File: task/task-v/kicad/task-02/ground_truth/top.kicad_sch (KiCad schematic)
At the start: 0 parts

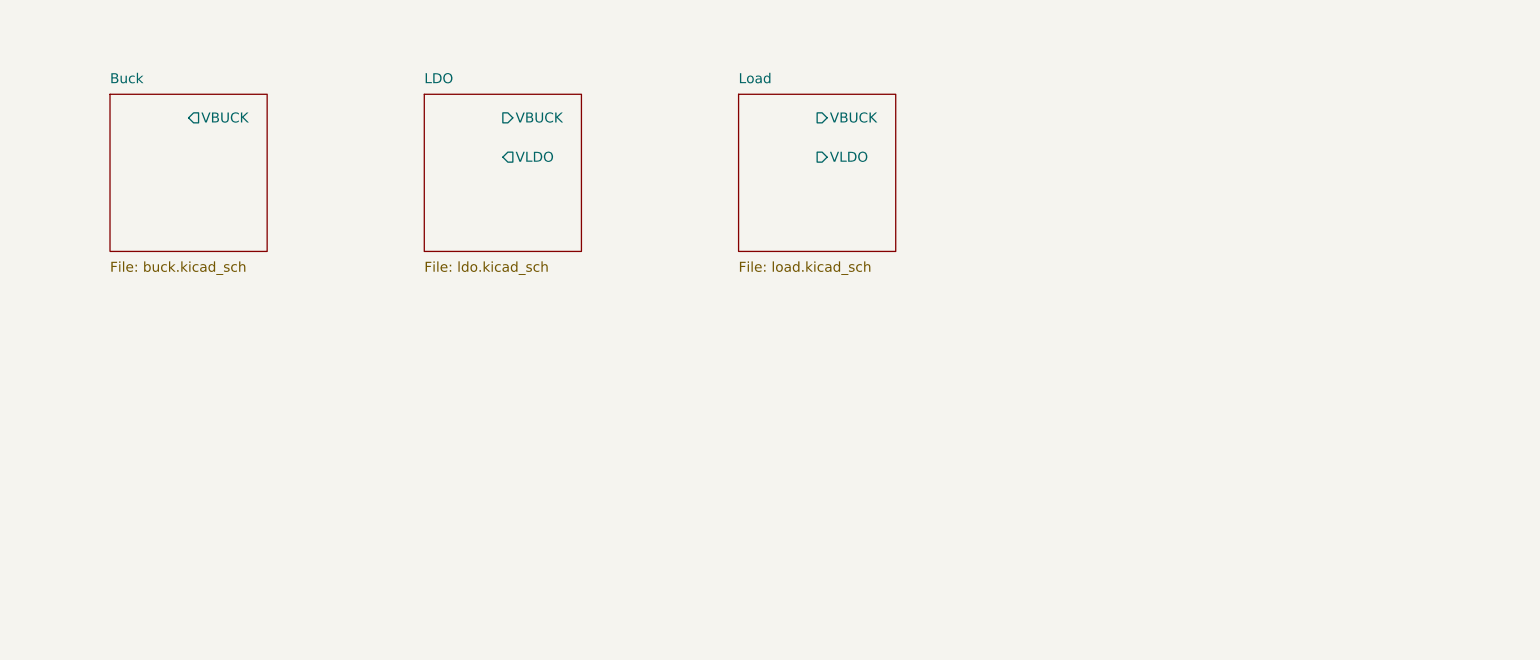
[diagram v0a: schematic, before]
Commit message: Repair KiCad 10.0.2 tasks and evaluators
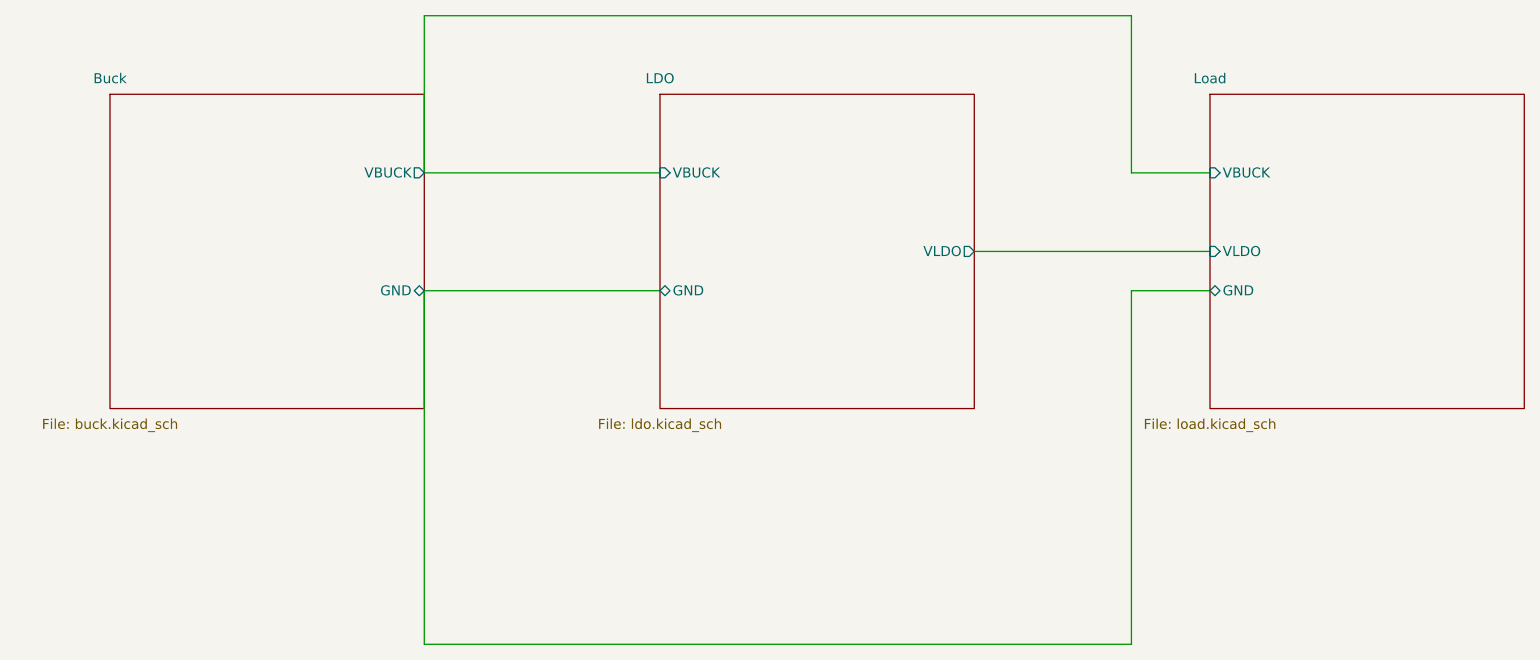
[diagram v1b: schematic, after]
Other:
- sheet Buck ports: added GND; removed none
- sheet LDO ports: added GND; removed none
- sheet Load ports: added GND; removed none
- company: SCH01 Benchmark -> EngiWorld
- title: Power Supply - Top Level -> Power Supply - Hierarchical Top
